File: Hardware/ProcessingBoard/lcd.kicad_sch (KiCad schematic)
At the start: 15 parts, among them J700 TXW280064B0, U700 CAT4139

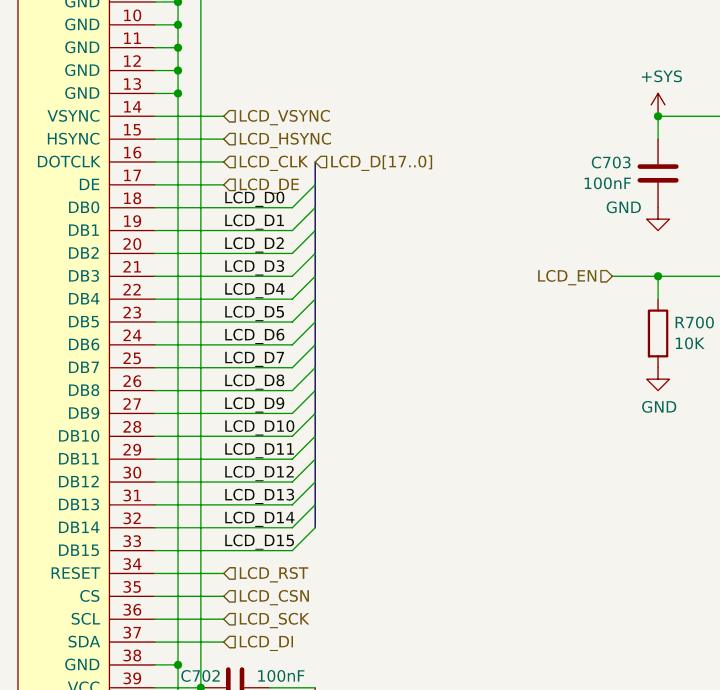
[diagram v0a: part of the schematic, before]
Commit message: Update License to match source code; test and fix USB, SEMC, and XIP on actual hardware
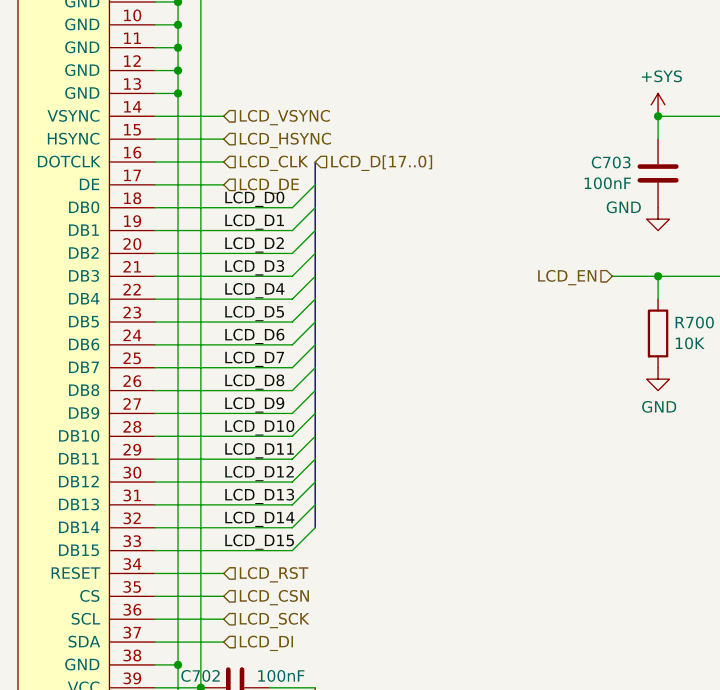
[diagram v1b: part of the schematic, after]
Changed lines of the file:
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@@
     (stroke (width 0) (type solid) (color 0 0 0 0))
   )
-  (bus (pts (xy 86.36 86.36) (xy 86.36 88.9))
+  (bus (pts (xy 86.36 86.36) (xy 86.36 127))
     (stroke (width 0) (type solid) (color 0 0 0 0))
   )
-  (bus (pts (xy 86.36 88.9) (xy 86.36 91.44))
-    (stroke (width 0) (type solid) (color 0 0 0 0))
-  )
-  (bus (pts (xy 86.36 91.44) (xy 86.36 93.98))
-    (stroke (width 0) (type solid) (color 0 0 0 0))
-  )
-  (bus (pts (xy 86.36 93.98) (xy 86.36 96.52))
-    (stroke (width 0) (type solid) (color 0 0 0 0))
-  )
-  (bus (pts (xy 86.36 96.52) (xy 86.36 99.06))
-    (stroke (width 0) (type solid) (color 0 0 0 0))
-  )
-  (bus (pts (xy 86.36 99.06) (xy 86.36 101.6))
-    (stroke (width 0) (type solid) (color 0 0 0 0))
-  )
-  (bus (pts (xy 86.36 101.6) (xy 86.36 104.14))
-    (stroke (width 0) (type solid) (color 0 0 0 0))
-  )
-  (bus (pts (xy 86.36 104.14) (xy 86.36 106.68))
-    (stroke (width 0) (type solid) (color 0 0 0 0))
-  )
-  (bus (pts (xy 86.36 106.68) (xy 86.36 109.22))
-    (stroke (width 0) (type solid) (color 0 0 0 0))
-  )
-  (bus (pts (xy 86.36 109.22) (xy 86.36 111.76))
-    (stroke (width 0) (type solid) (color 0 0 0 0))
-  )
-  (bus (pts (xy 86.36 111.76) (xy 86.36 114.3))
-    (stroke (width 0) (type solid) (color 0 0 0 0))
-  )
-  (bus (pts (xy 86.36 114.3) (xy 86.36 116.84))
-    (stroke (width 0) (type solid) (color 0 0 0 0))
-  )
-  (bus (pts (xy 86.36 116.84) (xy 86.36 119.38))
-    (stroke (width 0) (type solid) (color 0 0 0 0))
-  )
-  (bus (pts (xy 86.36 119.38) (xy 86.36 121.92))
-    (stroke (width 0) (type solid) (color 0 0 0 0))
-  )
-  (bus (pts (xy 86.36 121.92) (xy 86.36 124.46))
-    (stroke (width 0) (type solid) (color 0 0 0 0))
-  )
-  (bus (pts (xy 86.36 124.46) (xy 86.36 127))
-    (stroke (width 0) (type solid) (color 0 0 0 0))
-  )
